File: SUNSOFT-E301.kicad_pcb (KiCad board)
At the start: 2 copper layers, 92.1 x 57.1 mm, 27 parts, among them J1 Famicom Card Edge Connector, U1 HM6264, U2 FME7-5A-5B, U3 27C040, U4 27C020

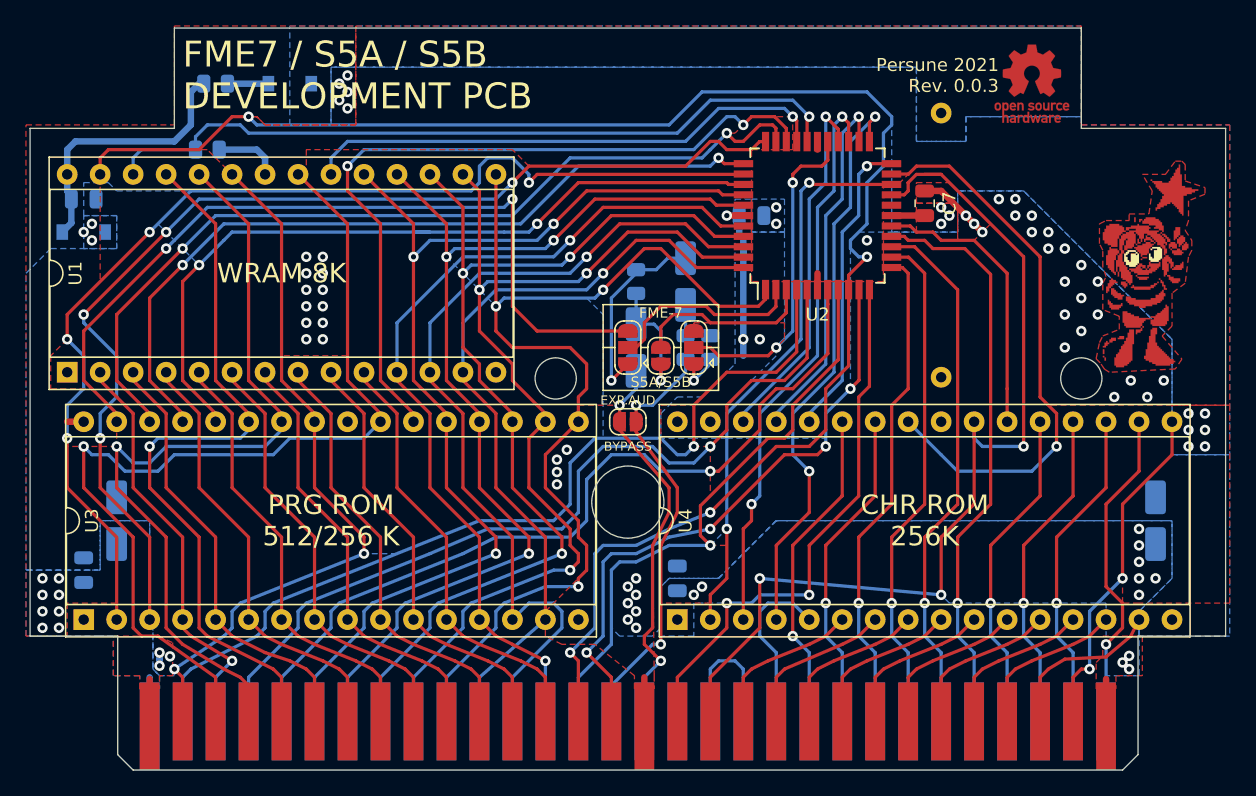
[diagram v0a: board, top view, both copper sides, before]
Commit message: Revision 0.0.4
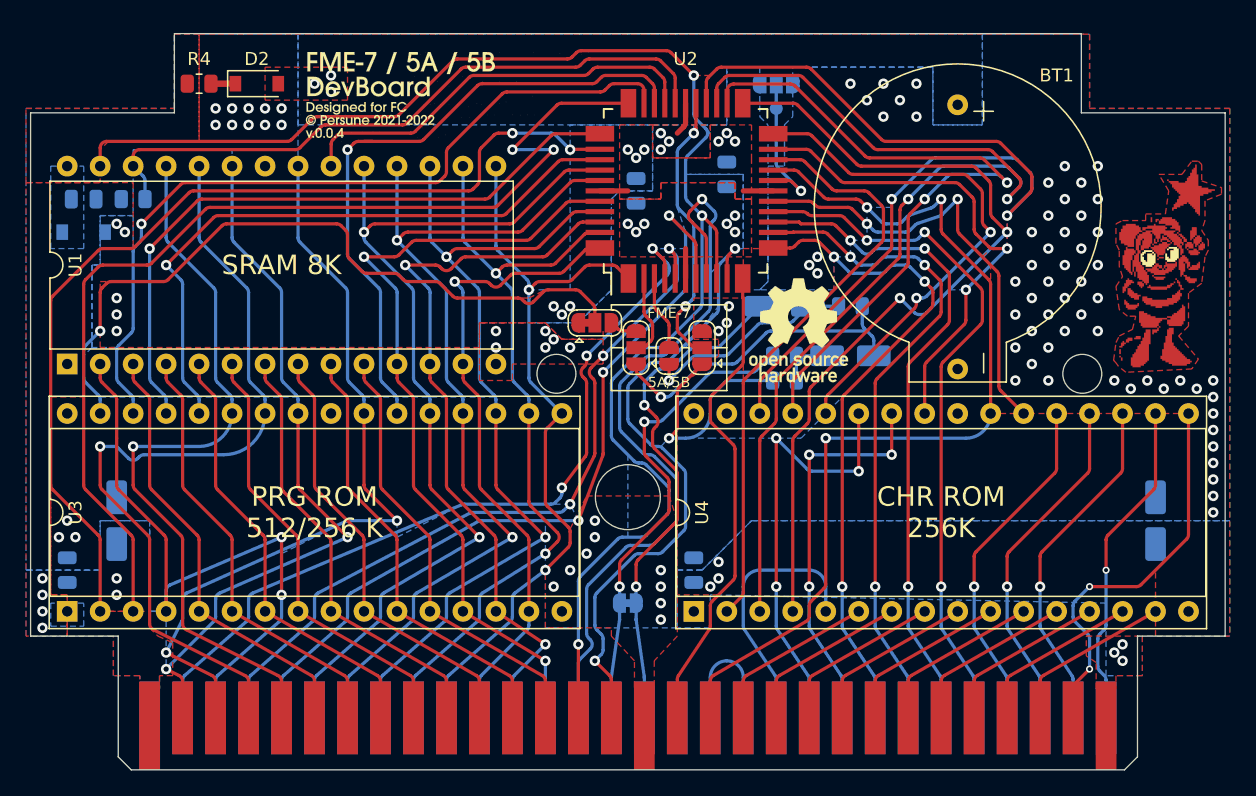
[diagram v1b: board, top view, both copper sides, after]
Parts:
- removed REF**: OSHW-Logo_5.7x6mm_Copper, Symbol:OSHW-Logo_5.7x6mm_Copper
- added JP5: ~, Jumper:SolderJumper-3_P1.3mm_Open_RoundedPad1.0x1.5mm, B.Cu at (163.8, 76.8)
- added JP6: ~, Jumper:SolderJumper-3_P1.3mm_Bridged12_RoundedPad1.0x1.5mm, F.Cu at (149.9, 95.2)
- added Ref**: Val**, custom footprints:art_front, F.Cu at (152.4, 101.3)
- added TP1: ~, TestPoint:TestPoint_Pad_D1.0mm, B.Cu at (163.8, 78.7)
- BT1, D2, R4: moved to F.Cu
- C7: moved to B.Cu
- JP1: value ~ -> SolderJumper_2_Bridged; footprint Jumper:SolderJumper-2_P1.3mm_Open_RoundedPad1.0x1.5mm -> Jumper:SolderJumper-2_P1.3mm_Bridged_RoundedPad1.0x1.5mm; moved to B.Cu
- U1: footprint Package_DIP:DIP-28_W15.24mm_Socket -> Package_DIP:DIP-28_W15.24mm
- U2: footprint Package_QFP:TQFP-44_10x10mm_P0.8mm -> custom footprints:Sunsoft-5
- moved R2 16.6 mm to (169.5, 94.0), turned to 180 degrees
- moved C7 15.4 mm to (160.0, 83.8), turned to -90 degrees
- moved JP1 14.0 mm to (152.4, 116.8)
- moved C2 13.9 mm to (169.5, 97.8), turned to 180 degrees
- moved C3 11.9 mm to (164.5, 94.0), turned to 180 degrees
- moved U2 10.3 mm to (156.8, 85.1), turned to 0 degrees
- moved C6 9.09 mm to (153.0, 85.1), turned to -90 degrees
- moved R3 7.65 mm to (164.5, 97.8), turned to 0 degrees
- moved R5 6.87 mm to (114.3, 85.7), turned to 180 degrees
- moved R1 6.25 mm to (164.5, 99.7), turned to 0 degrees
- moved D2 2.54 mm to (123.8, 76.8)
- moved BT1 1.42 mm to (177.8, 86.4)
- moved U3 1.42 mm to (109.2, 117.5)
- moved C5 1.42 mm to (157.5, 114.3)
- moved U4 1.42 mm to (157.5, 117.5)
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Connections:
- net Net-(BT1-Pad1) renamed /VCC_BATT
- J1 pad 47: Net-(J1-Pad47) -> unconnected-(J1-Pad47)
- JP1 pad 1: /AUD_IN -> /AUD_OUT
- JP1 pad 2: /AUD_OUT -> /AUD_IN
- JP2 pad 3: /PRG_A18 -> Net-(JP2-Pad3)
- U1 pad 1: Net-(U1-Pad1) -> unconnected-(U1-Pad1)
- U4 pad 31: Net-(U4-Pad31) -> unconnected-(U4-Pad31)
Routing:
- net /CHR_A17: track 28.4 -> 71.7 mm, vias 1 -> 2
- net /CHR_A15: track 44.0 -> 78.5 mm
- net /CHR_A14: track 28.1 -> 53.9 mm, vias 1 -> 2
- net /CPU_D3: track 81.7 -> 58.8 mm, vias 3 -> 2
- net Net-(C1-Pad2): track 20.2 -> 0.00 mm
- net VCC: track 24.5 -> 4.46 mm, vias 39 -> 29
- net /CHR_A12: track 45.0 -> 64.7 mm
- net /CPU_A12: track 31.4 -> 48.7 mm, vias 1 -> 2
- net /CHR_A13: track 23.5 -> 40.8 mm, vias 1 -> 2
- net /CPU_D4: track 76.8 -> 60.1 mm, vias 3 -> 2
- net GND: track 20.7 -> 4.85 mm, vias 52 -> 95
- net /S5B_AUD_OUT: track 3.39 -> 17.4 mm
- net /PPU_A10: track 37.4 -> 51.0 mm, vias 1 -> 3
- net /PPU_A11: track 38.4 -> 51.3 mm, vias 1 -> 3
- net /CPU_A10: track 72.8 -> 60.0 mm, vias 1 -> 2
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- added copper zone on F.Cu, net /VCC_BATT
- added copper zone on B.Cu, net Net-(C1-Pad2)
- added copper zone on F.Cu, net Net-(C1-Pad2)
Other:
- board size 92.1 x 57.1 mm -> 92 x 56.7 mm
- board text added: "5A/5B"
- board text added: "P.18 TEST"
- board text added: "SRAM 8K"
- board text added: "SS-E301 JxROM"
- board text removed: "FME7 / S5A / S5B DEVELOPMENT PCB"
- board text removed: "Persune 2021 Rev. 0.0.3"
- board text removed: "S5A/S5B"
- board text removed: "SS-E301"
- board text removed: "WRAM 8K"
